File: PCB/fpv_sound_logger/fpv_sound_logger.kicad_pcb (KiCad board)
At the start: 4 copper layers, 29.5 x 21.4 mm, 49 parts, among them CN1 SM04B-SRSS-TB(LF)(SN), IC1 W25Q128JVSIQ, J2 MSD-4-A, U2 INMP441ACEZ-R7, U3 TLV75533PDBVR, U4 SC0914_13_, Y1 ABM8-272-T3

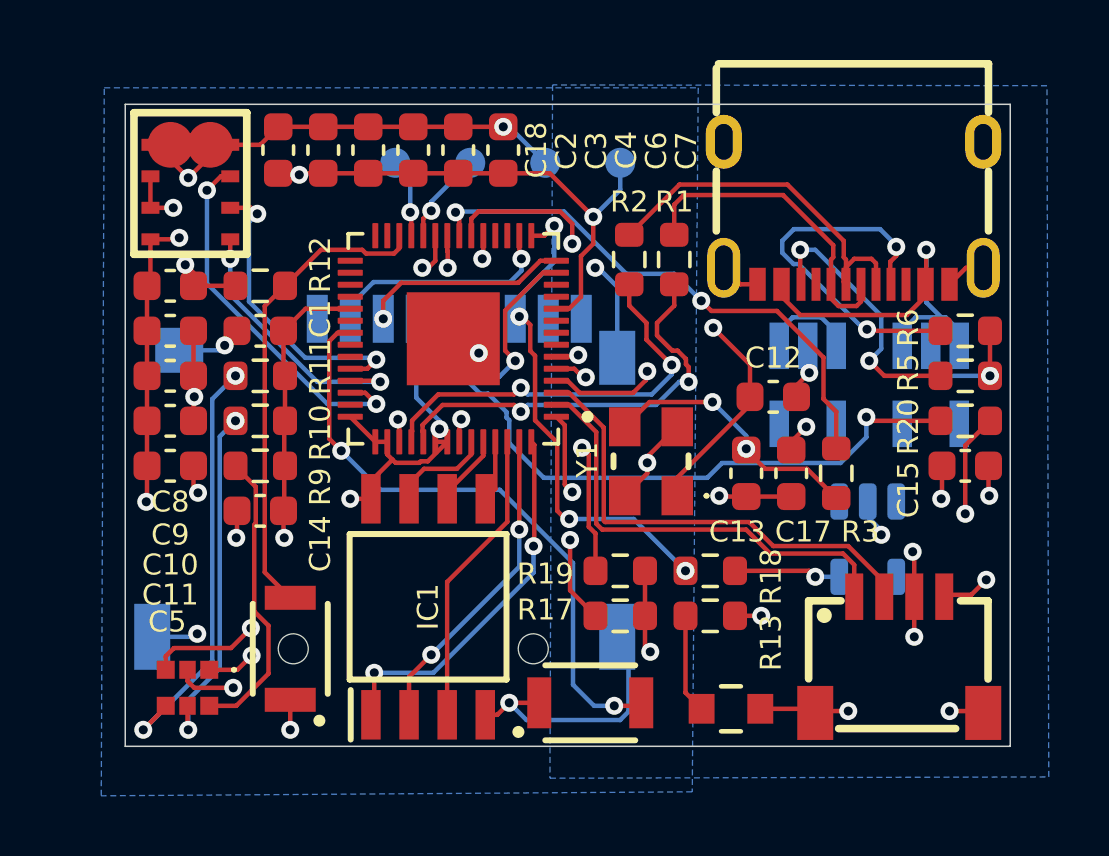
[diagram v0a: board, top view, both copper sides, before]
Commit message: Refactor code structure for improved readability and maintainability
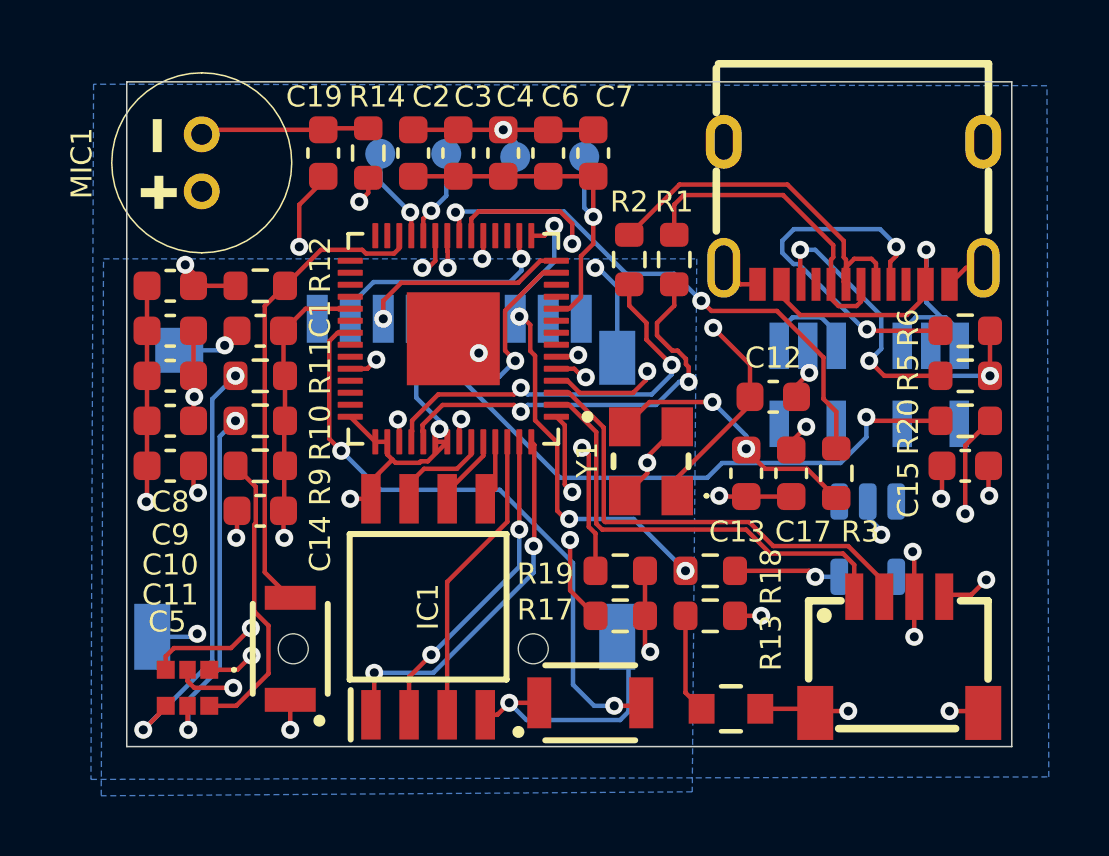
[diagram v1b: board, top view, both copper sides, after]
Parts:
- removed 3V3, CLK, DIO, GND: TestPoint, TestPoint:TestPoint_Pad_D1.0mm
- removed C18: 100n, Capacitor_SMD:C_0603_1608Metric
- removed U2: INMP441ACEZ-R7, fpv_sound_logger:MID-SMD_L4.7-W3.8_INMP441ACEZ
- added C19: 1u, Capacitor_SMD:C_0603_1608Metric, F.Cu at (131.1, 81.7)
- added MIC1: ~, fpv_sound_logger:MIC-TH_BD6.0-P1.90-D0.4-L-FD_GMI6050P-2CXXDB, F.Cu at (127.0, 82.0)
- added R14: 2k2, Resistor_SMD:R_0603_1608Metric, F.Cu at (132.6, 81.7)
- added TP1: TestPoint, TestPoint:TestPoint_Pad_D1.0mm, B.Cu at (135.2, 81.7)
- added TP2: TestPoint, TestPoint:TestPoint_Pad_D1.0mm, B.Cu at (133.0, 81.7)
- added TP3: TestPoint, TestPoint:TestPoint_Pad_D1.0mm, B.Cu at (137.5, 81.8)
- added TP4: TestPoint, TestPoint:TestPoint_Pad_D1.0mm, B.Cu at (139.8, 81.8)
- moved C2 3.00 mm to (134.1, 81.7)
- moved C3 3.00 mm to (135.6, 81.7)
- moved C4 3.00 mm to (137.1, 81.7)
- moved C6 3.00 mm to (138.6, 81.7)
- moved C7 3.00 mm to (140.1, 81.7)
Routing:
- net GPIO28_ADC2: track 12.4 -> 0.00 mm, vias 2 -> 0
- net GND: track 69.3 -> 59.8 mm, vias 22 -> 20
- net GPIO27_ADC1: track 9.07 -> 0.00 mm, vias 2 -> 0
- net +3V3: track 57.8 -> 51.8 mm, vias 14 -> 12
- net Net-(MIC1--): track 0.00 -> 5.63 mm
- net GPIO26_ADC0: track 10.1 -> 8.50 mm
- net +5V: track 3.56 -> 4.49 mm, vias 3 -> 4
- net SWD: track 2.65 -> 3.16 mm
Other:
- board size 29.5 x 21.4 mm -> 29.5 x 22.2 mm
